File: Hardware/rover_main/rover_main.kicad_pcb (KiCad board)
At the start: 2 copper layers, 85 x 70 mm, 36 parts, among them J1 BATT, J10 Analog, J2 BME280, J3 CSS811, J4 DRIVERS, J5 GY-87, J6 PROG, J7 FTDI, J8 Digital, U1 LD1117A33, U2 MCP732831CHARGER, U3 ESP32-CAM

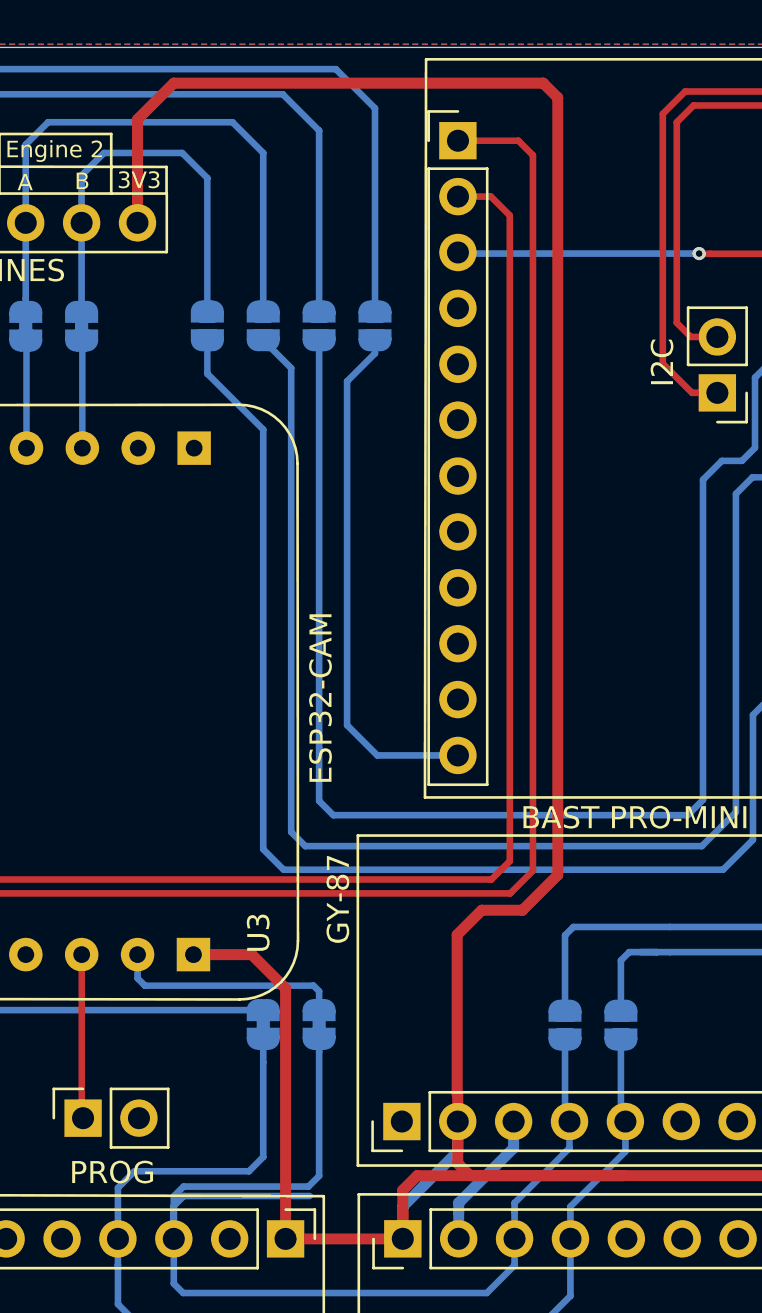
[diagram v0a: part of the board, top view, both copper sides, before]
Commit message: move  V track
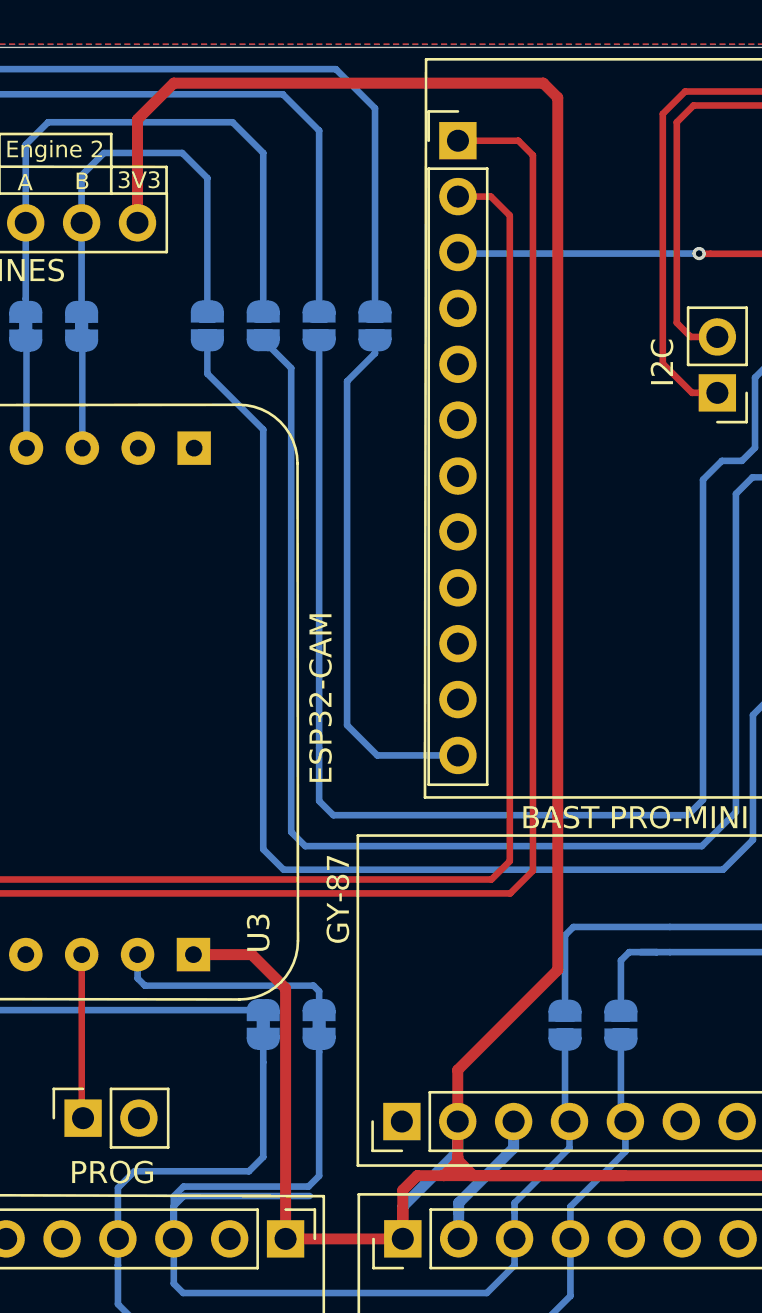
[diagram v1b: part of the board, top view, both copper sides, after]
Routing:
- net +3V3: track 205.3 -> 206.2 mm
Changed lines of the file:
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@@
     (thickness 1.6)
     (drawings 6343)
-    (tracks 305)
+    (tracks 308)
     (zones 0)
     (modules 36)
@@
   (segment (start 167.005 109.982) (end 167.005 111.252) (width 0.5) (layer F.Cu) (net 2))
   (segment (start 166.751 111.252) (end 166.497 111.506) (width 0.5) (layer F.Cu) (net 2))
-  (segment (start 147.27 108.92) (end 147.27 110.821) (width 0.5) (layer F.Cu) (net 2))
-  (segment (start 147.828 111.379) (end 149.86 111.379) (width 0.5) (layer F.Cu) (net 2))
-  (segment (start 147.27 110.821) (end 147.828 111.379) (width 0.5) (layer F.Cu) (net 2))
   (segment (start 144.769 114.254) (end 144.773 114.25) (width 0.5) (layer F.Cu) (net 2))
   (segment (start 139.445 114.254) (end 144.769 114.254) (width 0.5) (layer F.Cu) (net 2))
   (segment (start 144.773 114.25) (end 144.773 112.9) (width 0.5) (layer F.Cu) (net 2))
-  (segment (start 154.827 111.379) (end 145.431 111.379) (width 0.5) (layer F.Cu) (net 2))
   (segment (start 149.86 111.379) (end 154.827 111.379) (width 0.5) (layer F.Cu) (net 2))
   (segment (start 154.827 111.379) (end 165.989 111.379) (width 0.5) (layer F.Cu) (net 2))
@@
   (segment (start 164.7952 102.8954) (end 164.7952 106.1212) (width 0.5) (layer B.Cu) (net 2))
   (segment (start 164.7952 89.0778) (end 164.7952 102.8954) (width 0.5) (layer B.Cu) (net 2))
-  (segment (start 132.715 68.072) (end 132.715 63.373) (width 0.5) (layer F.Cu) (net 2))
-  (segment (start 132.715 63.373) (end 134.366 61.722) (width 0.5) (layer F.Cu) (net 2))
-  (segment (start 151.8158 97.7138) (end 151.8158 62.3824) (width 0.5) (layer F.Cu) (net 2))
-  (segment (start 150.2156 99.314) (end 151.8158 97.7138) (width 0.5) (layer F.Cu) (net 2))
-  (segment (start 134.366 61.722) (end 151.1554 61.722) (width 0.5) (layer F.Cu) (net 2))
-  (segment (start 147.27 108.92) (end 147.27 107.717919) (width 0.5) (layer F.Cu) (net 2))
-  (segment (start 148.3614 99.314) (end 150.2156 99.314) (width 0.5) (layer F.Cu) (net 2))
-  (segment (start 147.27 107.717919) (end 147.2438 107.691719) (width 0.5) (layer F.Cu) (net 2))
+  (segment (start 147.27 108.92) (end 147.27 106.5776) (width 0.5) (layer F.Cu) (net 2))
+  (segment (start 132.715 63.373) (end 132.715 68.072) (width 0.5) (layer F.Cu) (net 2))
+  (segment (start 147.27 106.5776) (end 151.8158 102.0318) (width 0.5) (layer F.Cu) (net 2))
+  (segment (start 151.8158 102.0318) (end 151.8158 62.3824) (width 0.5) (layer F.Cu) (net 2))
   (segment (start 151.8158 62.3824) (end 151.1554 61.722) (width 0.5) (layer F.Cu) (net 2))
-  (segment (start 147.2438 107.691719) (end 147.2438 100.4316) (width 0.5) (layer F.Cu) (net 2))
-  (segment (start 147.2438 100.4316) (end 148.3614 99.314) (width 0.5) (layer F.Cu) (net 2))
+  (segment (start 151.1554 61.722) (end 134.366 61.722) (width 0.5) (layer F.Cu) (net 2))
+  (segment (start 134.366 61.722) (end 132.715 63.373) (width 0.5) (layer F.Cu) (net 2))
+  (segment (start 147.1922 110.821) (end 146.6342 111.379) (width 0.5) (layer F.Cu) (net 2))
+  (segment (start 147.27 110.821) (end 147.1922 110.821) (width 0.5) (layer F.Cu) (net 2))
+  (segment (start 154.827 111.379) (end 146.6342 111.379) (width 0.5) (layer F.Cu) (net 2))
+  (segment (start 146.6342 111.379) (end 145.431 111.379) (width 0.5) (layer F.Cu) (net 2))
+  (segment (start 147.27 110.821) (end 147.828 111.379) (width 0.5) (layer F.Cu) (net 2))
+  (segment (start 147.27 110.6686) (end 147.9804 111.379) (width 0.5) (layer F.Cu) (net 2))
+  (segment (start 147.27 110.5146) (end 147.27 110.6686) (width 0.5) (layer F.Cu) (net 2))
+  (segment (start 147.9804 111.379) (end 149.86 111.379) (width 0.5) (layer F.Cu) (net 2))
+  (segment (start 147.828 111.379) (end 147.9804 111.379) (width 0.5) (layer F.Cu) (net 2))
+  (segment (start 147.27 110.5146) (end 147.27 110.821) (width 0.5) (layer F.Cu) (net 2))
+  (segment (start 147.27 108.92) (end 147.27 110.5146) (width 0.5) (layer F.Cu) (net 2))
   (segment (start 177.08 102) (end 178 102.92) (width 0.5) (layer B.Cu) (net 3))
   (segment (start 170 102) (end 177.08 102) (width 0.5) (layer B.Cu) (net 3))
